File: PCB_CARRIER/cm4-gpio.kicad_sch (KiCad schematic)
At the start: 28 parts, among them Q1 BSS138, Q2 BSS138, Q3 BSS138

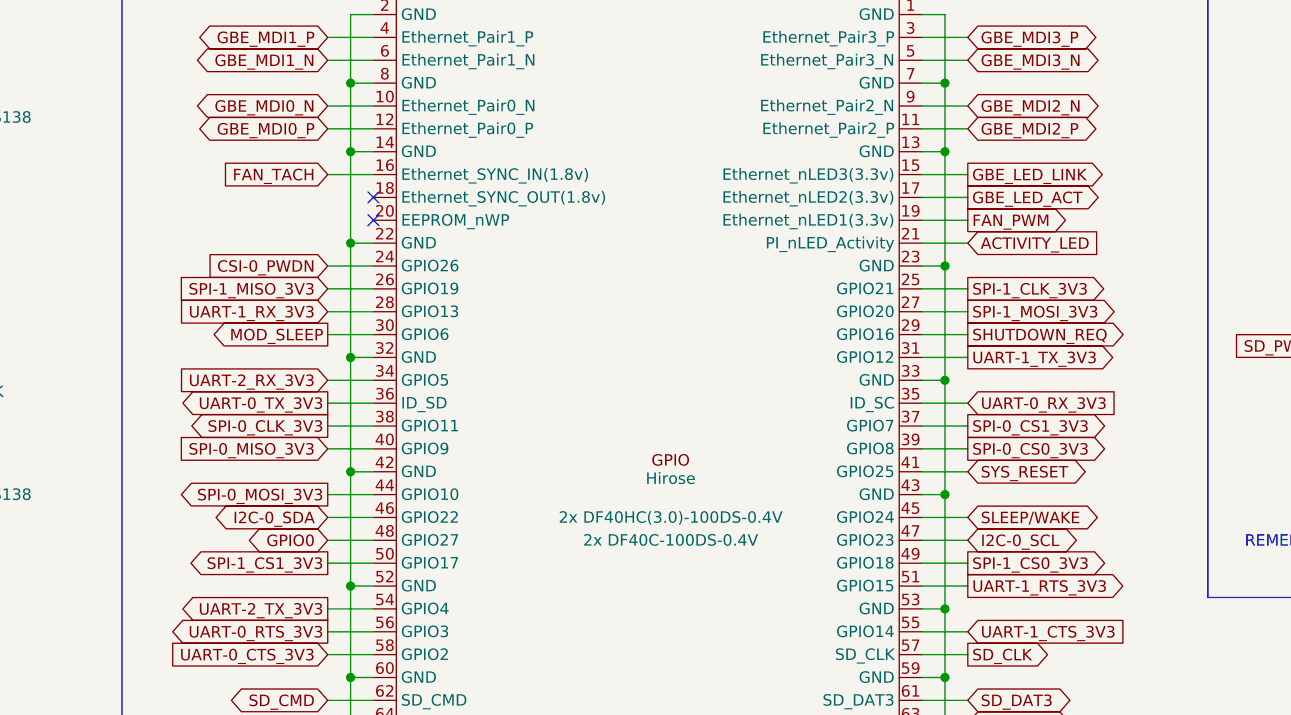
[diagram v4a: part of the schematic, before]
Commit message: only GPIO0 left to level shift, so I kinda wanna figure out a different way without adding a bidirectional shifter, but pwm and tach are in now
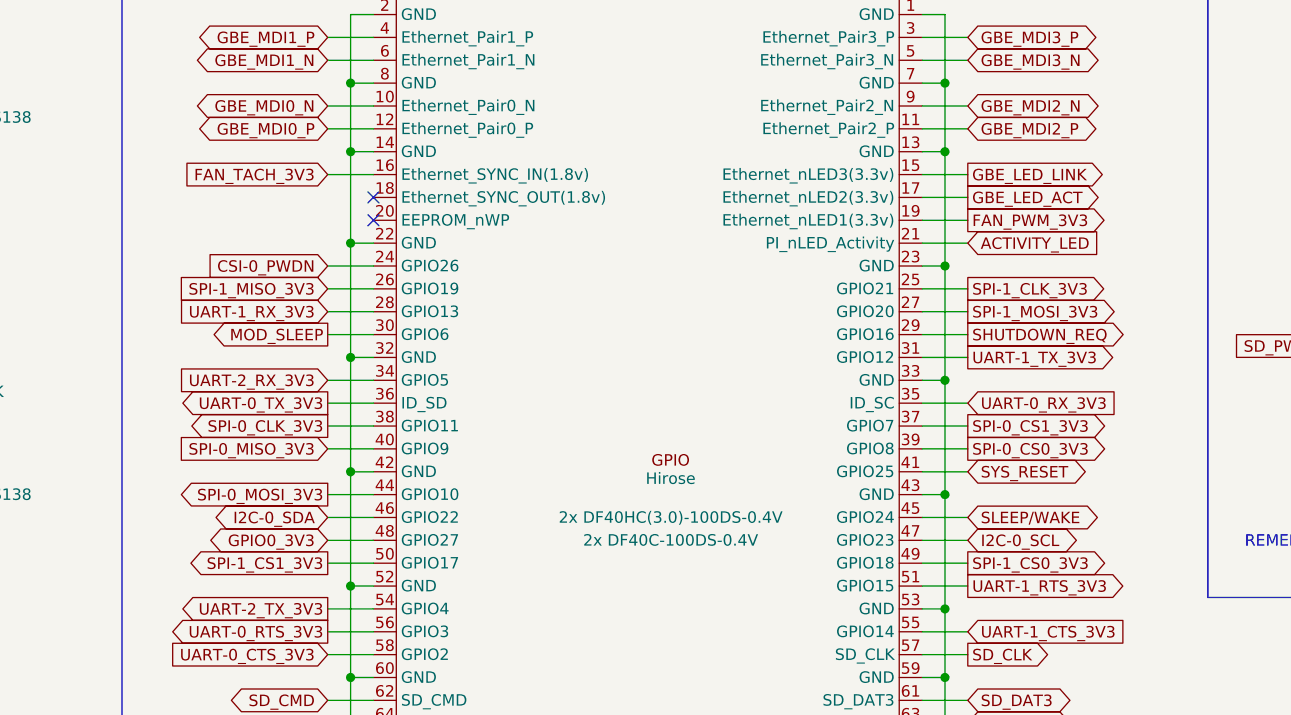
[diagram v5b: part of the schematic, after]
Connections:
- net FAN_PWM renamed FAN_PWM_3V3
- net FAN_TACH renamed FAN_TACH_3V3
- net GPIO0 renamed GPIO0_3V3
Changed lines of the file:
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@@
 		)
 	)
-	(global_label "GPIO0"
+	(global_label "GPIO0_3V3"
 		(shape bidirectional)
 		(at 100.33 87.63 180)
@@
 		)
 		(property "Intersheetrefs" "${INTERSHEET_REFS}"
-			(at 90.5489 87.63 0)
+			(at 86.0737 87.63 0)
 			(effects
 				(font
@@
 		)
 	)
-	(global_label "FAN_PWM"
+	(global_label "FAN_PWM_3V3"
 		(shape output)
 		(at 171.45 52.07 0)
@@
 		)
 		(property "Intersheetrefs" "${INTERSHEET_REFS}"
-			(at 183.1784 52.07 0)
+			(at 187.6536 52.07 0)
 			(effects
 				(font
@@
 		)
 	)
-	(global_label "FAN_TACH"
+	(global_label "FAN_TACH_3V3"
 		(shape input)
 		(at 100.33 46.99 180)
@@
 		)
 		(property "Intersheetrefs" "${INTERSHEET_REFS}"
-			(at 88.1177 46.99 0)
-			(effects
-				(font
+			(at 83.6425 46.99 0)
+			(effects
+				(font
